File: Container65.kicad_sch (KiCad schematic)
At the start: 25 parts

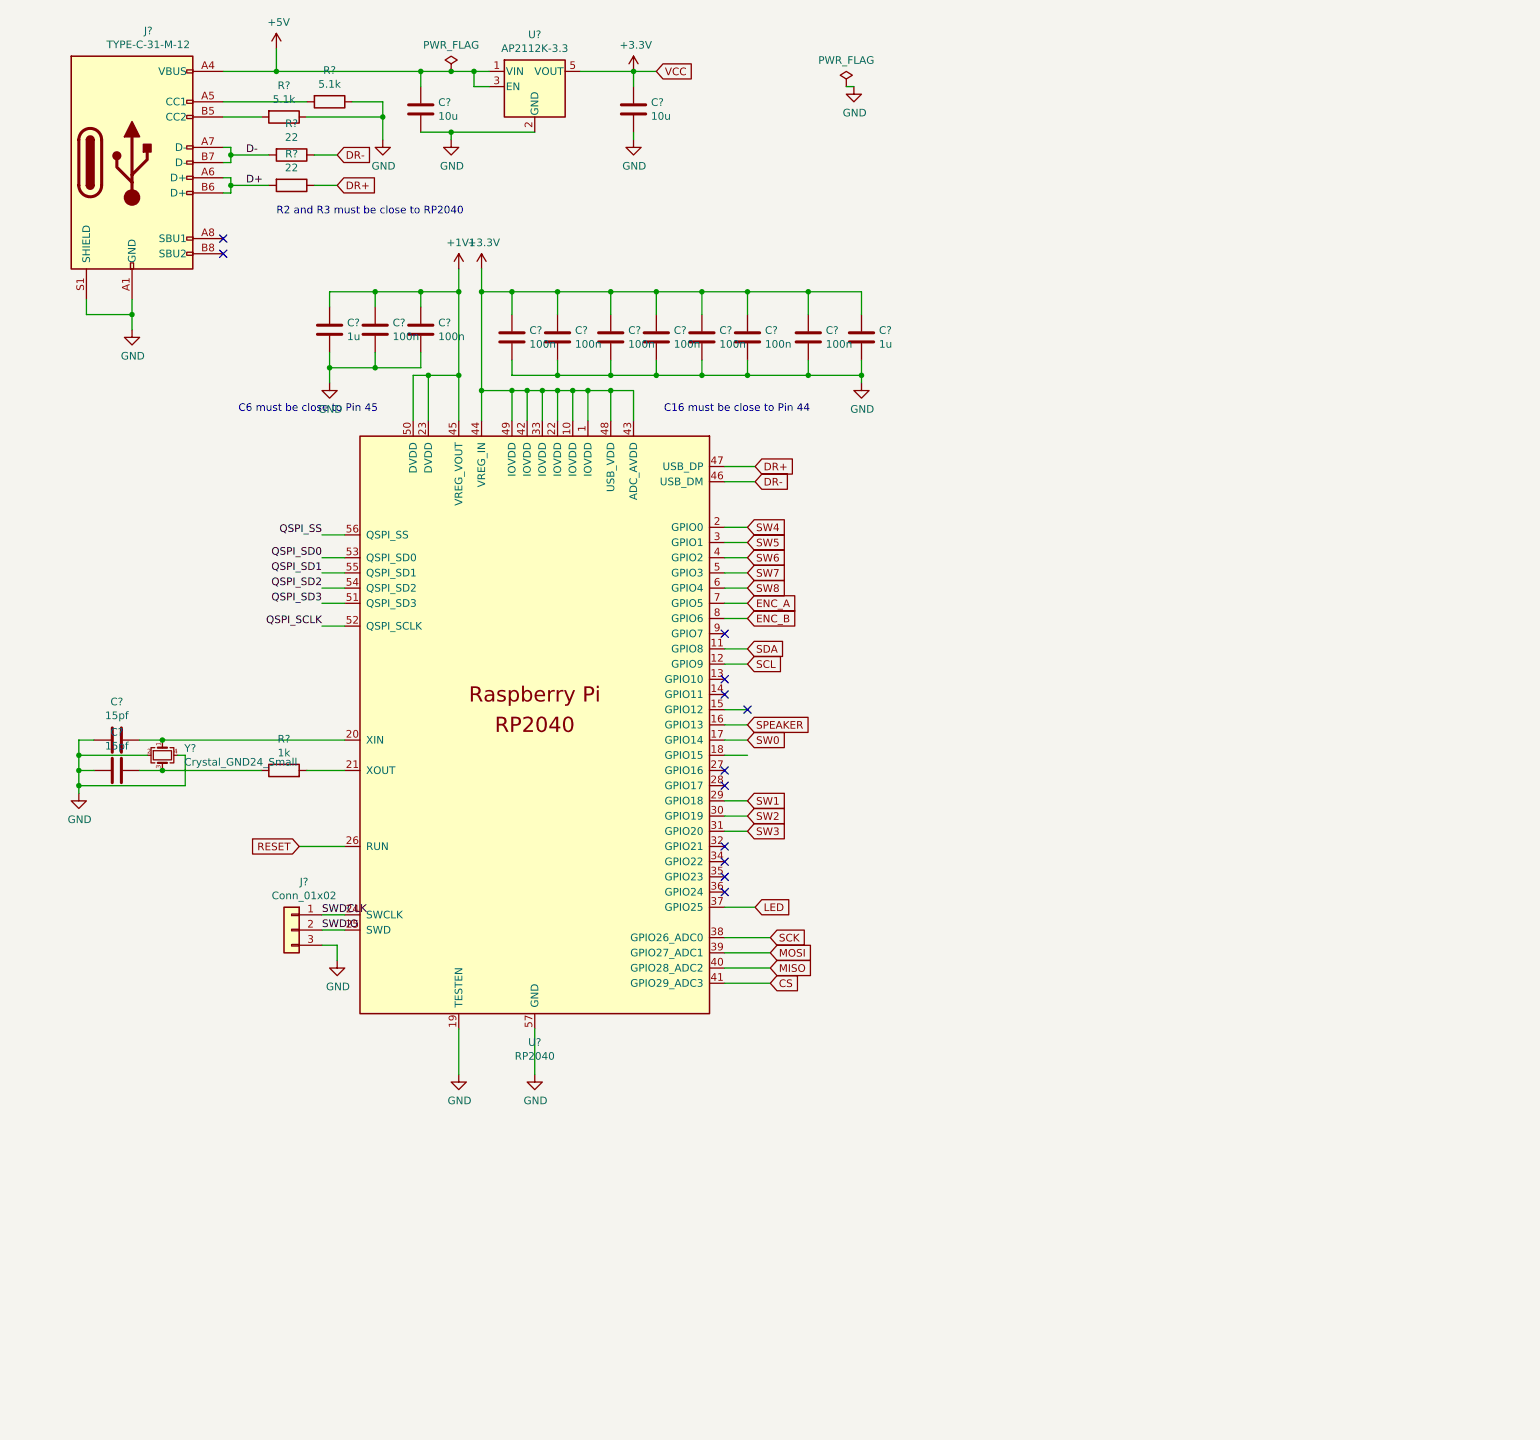
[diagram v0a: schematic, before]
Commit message: Matrix created
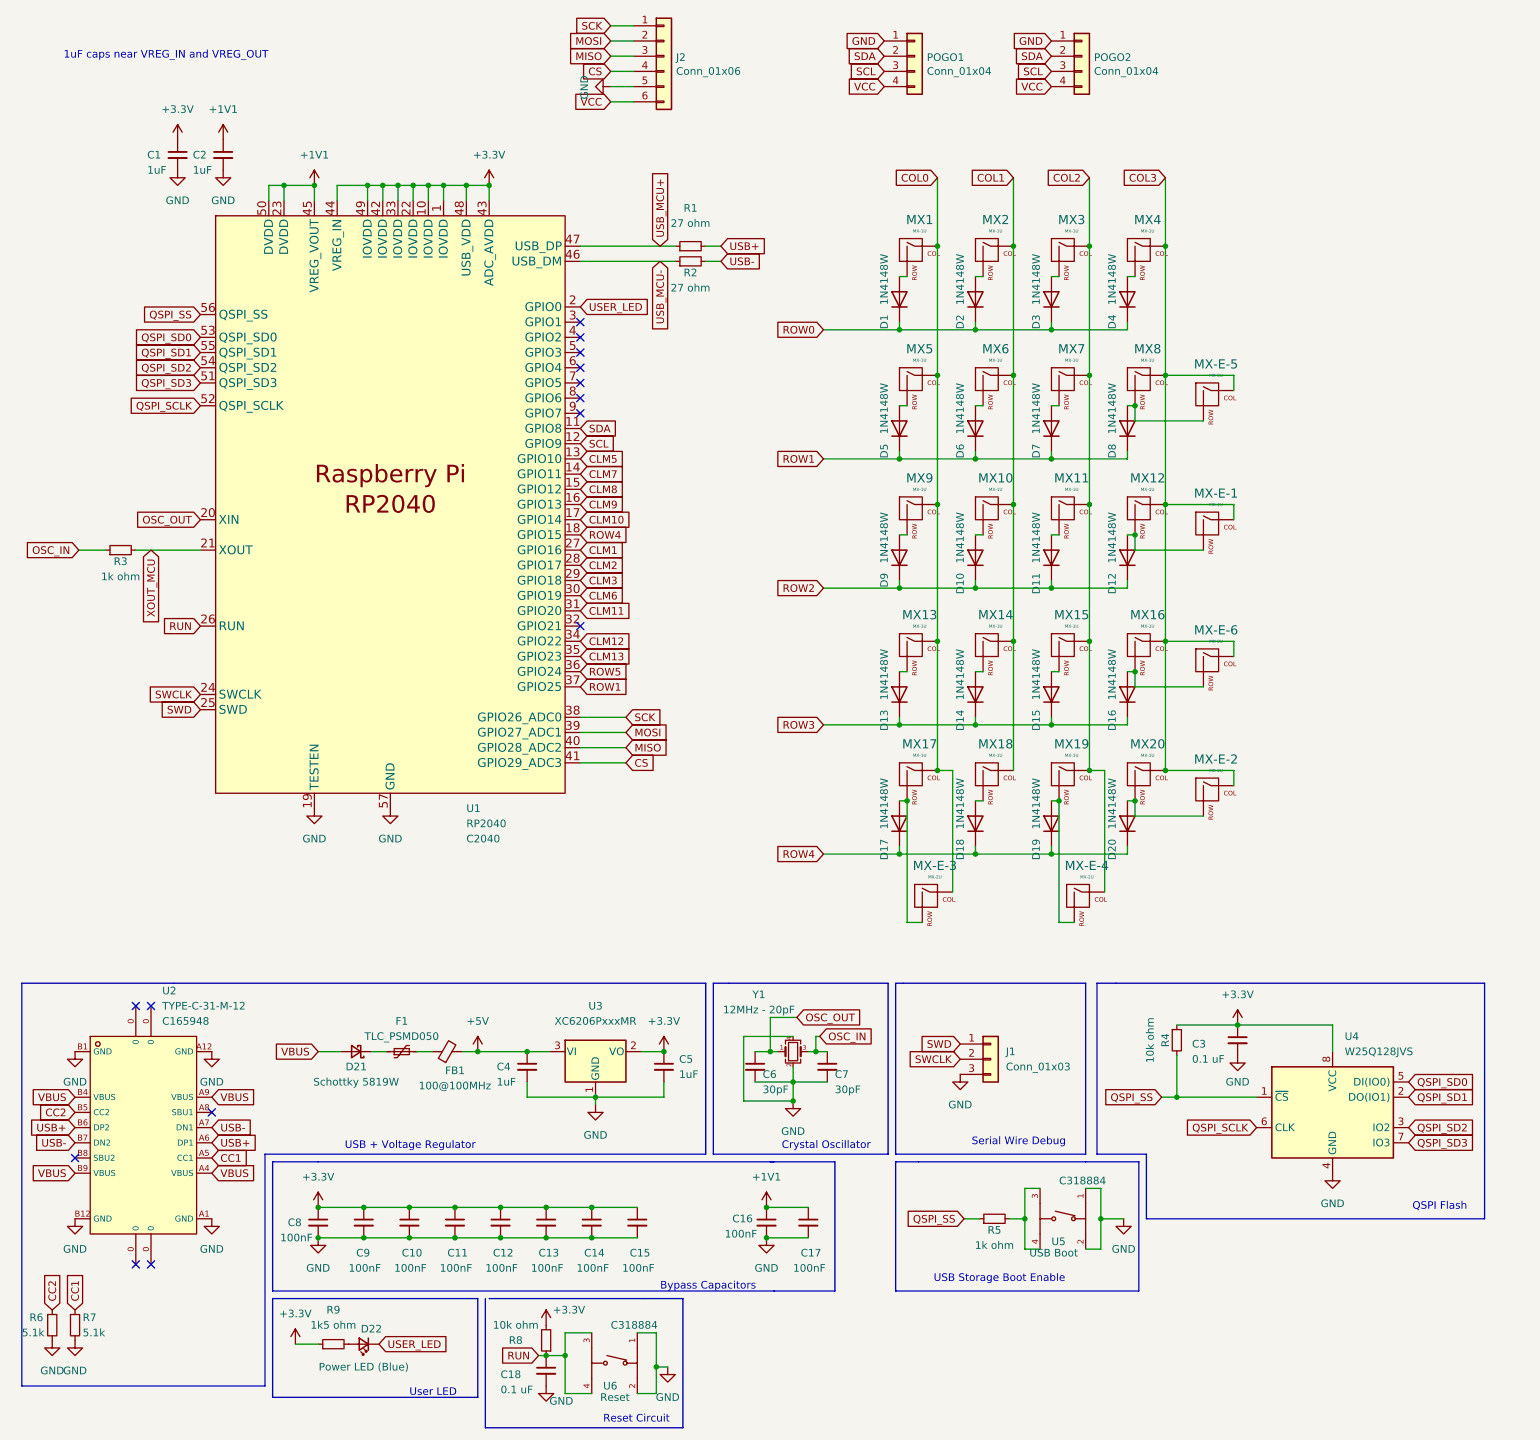
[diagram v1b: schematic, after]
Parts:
- removed C? (x9): 100n, Capacitor_SMD:C_0603_1608Metric, symbol Device:C
- removed C? (x2): 1u, Capacitor_SMD:C_0603_1608Metric, symbol Device:C
- removed C? (x2): 10u, Capacitor_SMD:C_0603_1608Metric, symbol Device:C
- removed C? (x2): 15pf, Capacitor_SMD:C_0603_1608Metric, symbol Device:C
- removed J?: TYPE-C-31-M-12, Connector_USB:USB_C_Receptacle_HRO_TYPE-C-31-M-12, symbol Connector:USB_C_Receptacle_USB2.0
- removed J?: Conn_01x02, Connector_PinHeader_2.54mm:PinHeader_1x03_P2.54mm_Vertical, symbol Connector_Generic:Conn_01x03
- removed R? (x2): 5.1k, Resistor_SMD:R_0603_1608Metric, symbol Device:R
- removed R? (x2): 22, Resistor_SMD:R_0603_1608Metric, symbol Device:R
- removed R?: 1k, Resistor_SMD:R_0603_1608Metric, symbol Device:R
- removed U?: RP2040, RP2040_minimal:RP2040-QFN-56, symbol MCU_RaspberryPi_RP2040:RP2040
- removed U?: AP2112K-3.3, Package_TO_SOT_SMD:SOT-23-5, symbol Regulator_Linear:AP2112K-3.3
- removed Y?: Crystal_GND24_Small, Crystal:Crystal_SMD_3225-4Pin_3.2x2.5mm, symbol Device:Crystal_GND24_Small
- added C1, C2, C4, C5: 1uF, Capacitor_SMD:C_0402_1005Metric, symbol Device:C_Small
- added C10, C11, C12, C13, C14, C15, C16, C17, C8, C9: 100nF, Capacitor_SMD:C_0402_1005Metric, symbol Device:C_Small
- added C18, C3: 0.1 uF, Capacitor_SMD:C_0402_1005Metric, symbol Device:C_Small
- added C6, C7: 30pF, Capacitor_SMD:C_0402_1005Metric, symbol Device:C_Small
- added D1, D10, D11, D12, D13, D14, D15, D16, D17, D18, D19, D2, D20, D3, D4, D5, D6, D7, D8, D9: 1N4148W, Diode_SMD:D_SOD-123, symbol Diode:1N4148W
- added D21: Schottky 5819W, Diode_SMD:D_SOD-123, symbol Device:D_Schottky_Small
- added D22: Power LED (Blue), LED_SMD:LED_0805_2012Metric, symbol Device:LED_Small
- added F1: TLC_PSMD050, Fuse:Fuse_0805_2012Metric, symbol Device:Polyfuse_Small
- added FB1: 100@100MHz, Inductor_SMD:L_0805_2012Metric, symbol Device:FerriteBead_Small
- added J1: Conn_01x03, Connector_PinHeader_2.54mm:PinHeader_1x03_P2.54mm_Vertical, symbol Connector_Generic:Conn_01x03
- added J2: Conn_01x06, Connector_PinHeader_1.27mm:PinHeader_1x06_P1.27mm_Vertical, symbol Connector_Generic:Conn_01x06
- added MX-E-1, MX-E-2, MX-E-3, MX-E-4, MX-E-5, MX-E-6: MX-2U, MX_Only:MXOnly-1U-NoLEDHotswap, symbol MX_Alps_Hybrid:MX-NoLED
- added MX1, MX10, MX11, MX12, MX13, MX14, MX15, MX16, MX17, MX18, MX19, MX2, MX20, MX3, MX4, MX5, MX6, MX7, MX8, MX9: MX-1U, MX_Only:MXOnly-1U-NoLEDHotswap, symbol MX_Alps_Hybrid:MX-NoLED
- added POGO1: Conn_01x04, 65Numpad:PogoConnector, symbol Connector_Generic:Conn_01x04
- added POGO2: Conn_01x04, 65Numpad:PogoConnectorMirrored, symbol Connector_Generic:Conn_01x04
- added R1, R2: 27 ohm, Resistor_SMD:R_0603_1608Metric, symbol Device:R_Small
- added R3, R5: 1k ohm, Resistor_SMD:R_0402_1005Metric, symbol Device:R_Small
- added R4, R8: 10k ohm, Resistor_SMD:R_0402_1005Metric, symbol Device:R_Small
- added R6, R7: 5.1k, Resistor_SMD:R_0402_1005Metric, symbol Device:R_Small
- added R9: 1k5 ohm, Resistor_SMD:R_0402_1005Metric, symbol Device:R_Small
- added U1: RP2040, footprints:rp2040, symbol rp2040:RP2040
- added U2: TYPE-C-31-M-12, footprints:simple-usb-c, symbol simple-usb-c:TYPE-C-31-M-12
- added U3: XC6206PxxxMR, Package_TO_SOT_SMD:SOT-23, symbol Regulator_Linear:XC6206PxxxMR
- added U4: W25Q128JVS, Package_SO:SOIC-8_5.23x5.23mm_P1.27mm, symbol Memory_Flash:W25Q128JVS
- added U5: USB Boot, footprints:tactile-switch, symbol tactile-switch:TS-1187A-B-A-B
- added U6: Reset, footprints:tactile-switch, symbol tactile-switch:TS-1187A-B-A-B
- added Y1: 12MHz - 20pF, Crystal:Crystal_SMD_3225-4Pin_3.2x2.5mm, symbol Device:Crystal_GND24_Small
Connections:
- net +1V1: now also C16.1, C17.1, C2.1, U1.23 (DVDD), U1.45 (VREG_VOUT), U1.50 (DVDD)
- net +3V3: now also C1.1, C10.1, C11.1, C12.1, C13.1, C14.1, C15.1, C3.1, C5.1, C8.1, C9.1, R4.1, R8.2, R9.1, U1.1 (IOVDD), U1.10 (IOVDD), U1.22 (IOVDD), U1.33 (IOVDD), U1.42 (IOVDD), U1.43 (ADC_AVDD), U1.44 (VREG_IN), U1.48 (USB_VDD), U1.49 (IOVDD), U3.2 (VO), U4.8 (VCC)
- net +5V: now also C4.1, FB1.2, U3.3 (VI)
- net CS: now also J2.4 (Pin_4), U1.41 (GPIO29_ADC3)
- net GND: now also C1.2, C10.2, C11.2, C12.2, C13.2, C14.2, C15.2, C16.2, C17.2, C18.2, C2.2, C3.2, C4.2, C5.2, C6.2, C7.2, C8.2, C9.2, J1.3 (Pin_3), J2.5 (Pin_5), POGO1.1 (Pin_1), POGO2.1 (Pin_1), R6.2, R7.2, U1.19 (TESTEN), U1.57 (GND), U2.A1 (GND), U2.A12 (GND), U2.B1 (GND), U2.B12 (GND), U3.1 (GND), U4.4 (GND), U5.1 (A), U5.2 (B), U6.1 (A), U6.2 (B), Y1.2, Y1.4
- net MISO: now also J2.3 (Pin_3), U1.40 (GPIO28_ADC2)
- net MOSI: now also J2.2 (Pin_2), U1.39 (GPIO27_ADC1)
- net QSPI_SCLK: now also U1.52 (QSPI_SCLK), U4.6 (CLK)
- net QSPI_SD0: now also U1.53 (QSPI_SD0), U4.5 (DI(IO0))
- net QSPI_SD1: now also U1.55 (QSPI_SD1), U4.2 (DO(IO1))
- net QSPI_SD2: now also U1.54 (QSPI_SD2), U4.3 (IO2)
- net QSPI_SD3: now also U1.51 (QSPI_SD3), U4.7 (IO3)
- net QSPI_SS: now also R4.2, R5.1, U1.56 (QSPI_SS), U4.1 (~{CS})
- net SCK: now also J2.1 (Pin_1), U1.38 (GPIO26_ADC0)
- net SCL: now also POGO1.3 (Pin_3), POGO2.3 (Pin_3), U1.12 (GPIO9)
- net SDA: now also POGO1.2 (Pin_2), POGO2.2 (Pin_2), U1.11 (GPIO8)
- new net: D20.2 (A), MX-E-2.2 (ROW), MX20.2 (ROW)
- new net: D17.2 (A), MX-E-3.2 (ROW), MX17.2 (ROW)
- new net: D19.2 (A), MX-E-4.2 (ROW), MX19.2 (ROW)
- new net: D21.1 (K), F1.1
- new net: F1.2, FB1.1
- new net: D8.2 (A), MX-E-5.2 (ROW), MX8.2 (ROW)
- new net: D9.2 (A), MX9.2 (ROW)
- new net: D3.2 (A), MX3.2 (ROW)
- new net: D1.2 (A), MX1.2 (ROW)
- new net: D22.2 (A), R9.2
- new net: D18.2 (A), MX18.2 (ROW)
- new net: D16.2 (A), MX-E-6.2 (ROW), MX16.2 (ROW)
- new net: D10.2 (A), MX10.2 (ROW)
- new net: D11.2 (A), MX11.2 (ROW)
- new net: D2.2 (A), MX2.2 (ROW)
- new net: D13.2 (A), MX13.2 (ROW)
- new net: D6.2 (A), MX6.2 (ROW)
- new net: D4.2 (A), MX4.2 (ROW)
- new net: D12.2 (A), MX-E-1.2 (ROW), MX12.2 (ROW)
- new net: R5.2, U5.3 (C), U5.4 (D)
- new net: D15.2 (A), MX15.2 (ROW)
- new net: D7.2 (A), MX7.2 (ROW)
- new net: D14.2 (A), MX14.2 (ROW)
- new net: D5.2 (A), MX5.2 (ROW)
- new net CC1: R7.1, U2.A5 (CC1)
- new net CC2: R6.1, U2.B5 (CC2)
- new net CLM1: U1.27 (GPIO16)
- new net CLM10: U1.17 (GPIO14)
- new net CLM11: U1.31 (GPIO20)
- new net CLM12: U1.34 (GPIO22)
- new net CLM13: U1.35 (GPIO23)
- new net CLM2: U1.28 (GPIO17)
- new net CLM3: U1.29 (GPIO18)
- new net CLM5: U1.13 (GPIO10)
- new net CLM6: U1.30 (GPIO19)
- new net CLM7: U1.14 (GPIO11)
- new net CLM8: U1.15 (GPIO12)
- new net CLM9: U1.16 (GPIO13)
- new net COL0: MX-E-3.1 (COL), MX1.1 (COL), MX13.1 (COL), MX17.1 (COL), MX5.1 (COL), MX9.1 (COL)
- new net COL1: MX10.1 (COL), MX14.1 (COL), MX18.1 (COL), MX2.1 (COL), MX6.1 (COL)
- new net COL2: MX-E-4.1 (COL), MX11.1 (COL), MX15.1 (COL), MX19.1 (COL), MX3.1 (COL), MX7.1 (COL)
- new net COL3: MX-E-1.1 (COL), MX-E-2.1 (COL), MX-E-5.1 (COL), MX-E-6.1 (COL), MX12.1 (COL), MX16.1 (COL), MX20.1 (COL), MX4.1 (COL), MX8.1 (COL)
- new net OSC_IN: C7.1, R3.1, Y1.3
- new net OSC_OUT: C6.1, U1.20 (XIN), Y1.1
- new net ROW0: D1.1 (K), D2.1 (K), D3.1 (K), D4.1 (K)
- new net ROW1: D5.1 (K), D6.1 (K), D7.1 (K), D8.1 (K), U1.37 (GPIO25)
- new net ROW2: D10.1 (K), D11.1 (K), D12.1 (K), D9.1 (K)
- new net ROW3: D13.1 (K), D14.1 (K), D15.1 (K), D16.1 (K)
- new net ROW4: D17.1 (K), D18.1 (K), D19.1 (K), D20.1 (K), U1.18 (GPIO15)
- new net ROW5: U1.36 (GPIO24)
- new net RUN: C18.1, R8.1, U1.26 (RUN), U6.3 (C), U6.4 (D)
- new net SWCLK: J1.2 (Pin_2), U1.24 (SWCLK)
- new net SWD: J1.1 (Pin_1), U1.25 (SWD)
- new net USB+: R1.2, U2.A6 (DP1), U2.B6 (DP2)
- new net USB-: R2.2, U2.A7 (DN1), U2.B7 (DN2)
- new net USB_MCU+: R1.1, U1.47 (USB_DP)
- new net USB_MCU-: R2.1, U1.46 (USB_DM)
- new net USER_LED: D22.1 (K), U1.2 (GPIO0)
- new net VBUS: D21.2 (A), U2.A4 (VBUS), U2.A9 (VBUS), U2.B4 (VBUS), U2.B9 (VBUS)
- new net VCC: J2.6 (Pin_6), POGO1.4 (Pin_4), POGO2.4 (Pin_4)
- new net XOUT_MCU: R3.2, U1.21 (XOUT)
- no-connect marks 12 -> 14
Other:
- note added: "1uF caps near VREG_IN and VREG_OUT"
- note added: "Bypass Capacitors"
- note added: "Crystal Oscillator"
- note added: "QSPI Flash"
- note added: "Reset Circuit"
- note added: "Serial Wire Debug"
- note added: "USB + Voltage Regulator"
- note added: "USB Storage Boot Enable"
- note added: "User LED"
- note removed: "C16 must be close to Pin 44"
- note removed: "C6 must be close to Pin 45"
- note removed: "R2 and R3 must be close to RP2040"
